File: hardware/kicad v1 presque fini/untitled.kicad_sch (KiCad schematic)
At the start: 38 parts, among them IC2 LDO40LPU33RY, IC3 L7981TR, IC4 TSC102IDT, IC5 LDO40LPU33RY, J11 connecteur uart, J3 connecteur gps, J4 connecteur radio, J5 connecteur uart, J7 connecteur swd, J8 connecteur servo

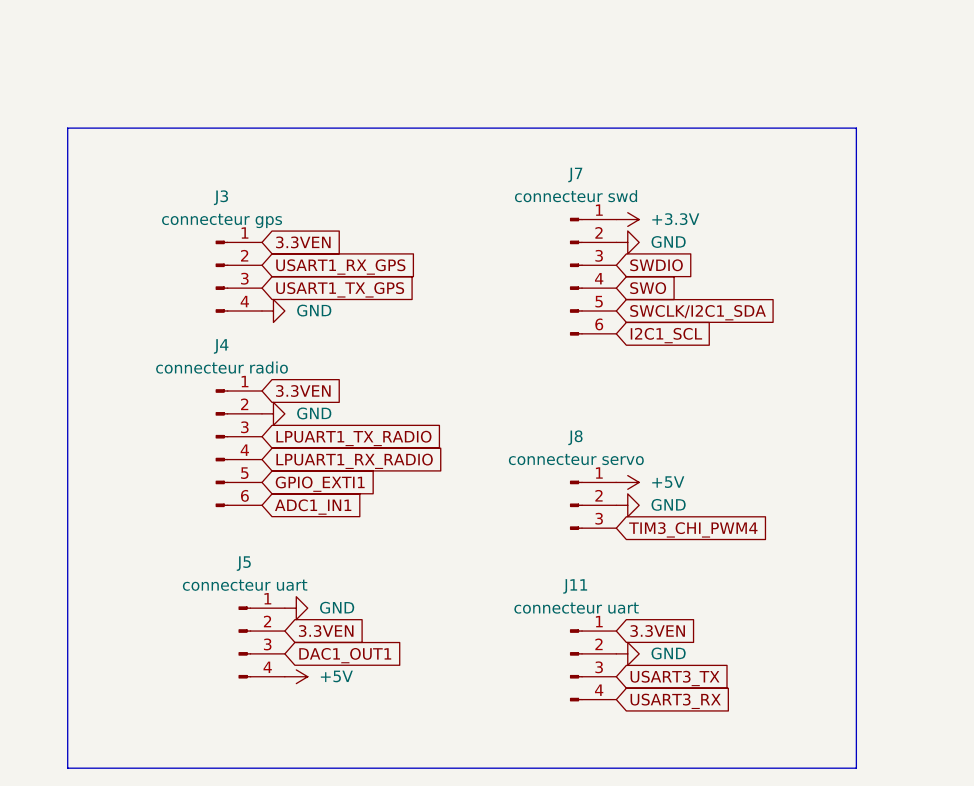
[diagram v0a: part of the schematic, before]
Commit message: pcb
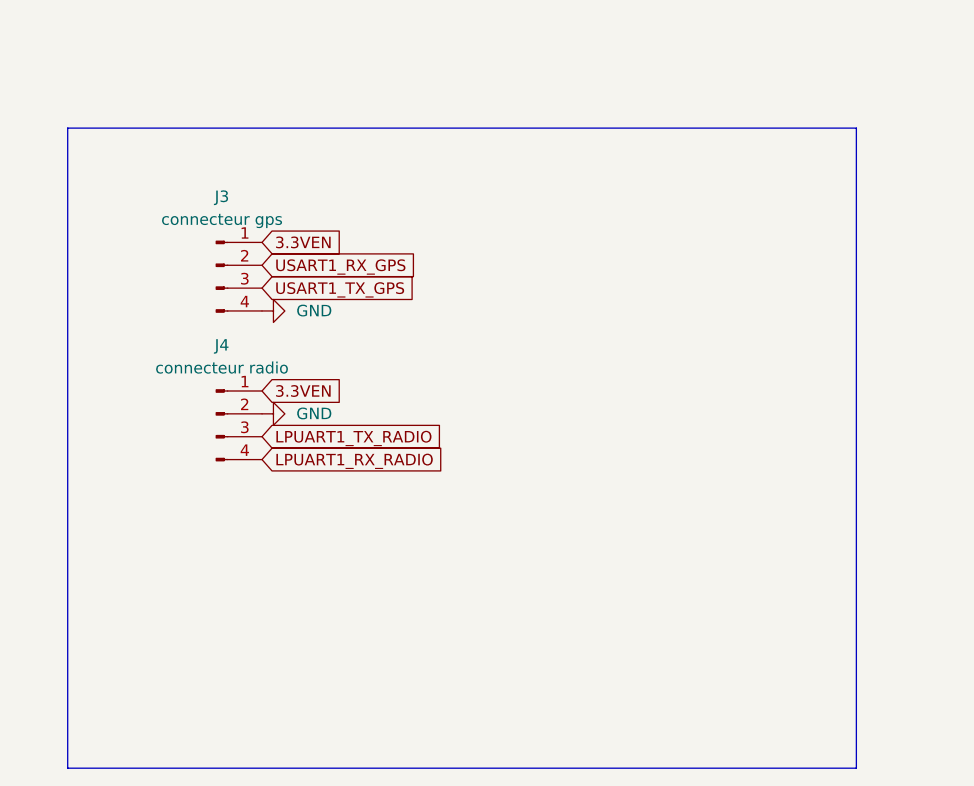
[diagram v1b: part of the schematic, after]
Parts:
- removed J11, J5: connecteur uart, Connector_JST:JST_SH_BM04B-SRSS-TB_1x04-1MP_P1.00mm_Vertical, symbol Connector:Conn_01x04_Pin
- removed J4: connecteur radio, Connector_JST:JST_SH_BM06B-SRSS-TB_1x06-1MP_P1.00mm_Vertical, symbol Connector:Conn_01x06_Pin
- removed J7: connecteur swd, Connector_JST:JST_SH_BM06B-SRSS-TB_1x06-1MP_P1.00mm_Vertical, symbol Connector:Conn_01x06_Pin
- removed J8: connecteur servo, Connector_JST:JST_SH_BM03B-SRSS-TB_1x03-1MP_P1.00mm_Vertical, symbol Connector:Conn_01x03_Pin
- added J4: connecteur radio, Connector_JST:JST_SH_BM04B-SRSS-TB_1x04-1MP_P1.00mm_Vertical, symbol Connector:Conn_01x04_Pin
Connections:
- net 3.3VEN: now also J4.1 (Pin_1)
- net GND: now also J4.2 (Pin_2)
- net LPUART1_RX_RADIO: now also J4.4 (Pin_4)
- net LPUART1_TX_RADIO: now also J4.3 (Pin_3)
